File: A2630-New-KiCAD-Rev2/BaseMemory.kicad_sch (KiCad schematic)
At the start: 13 parts, among them U300 74HCT05, U400 SDRAM_32Mb(2Mx16), U401 SDRAM_32Mb(2Mx16), U606 74HCT244

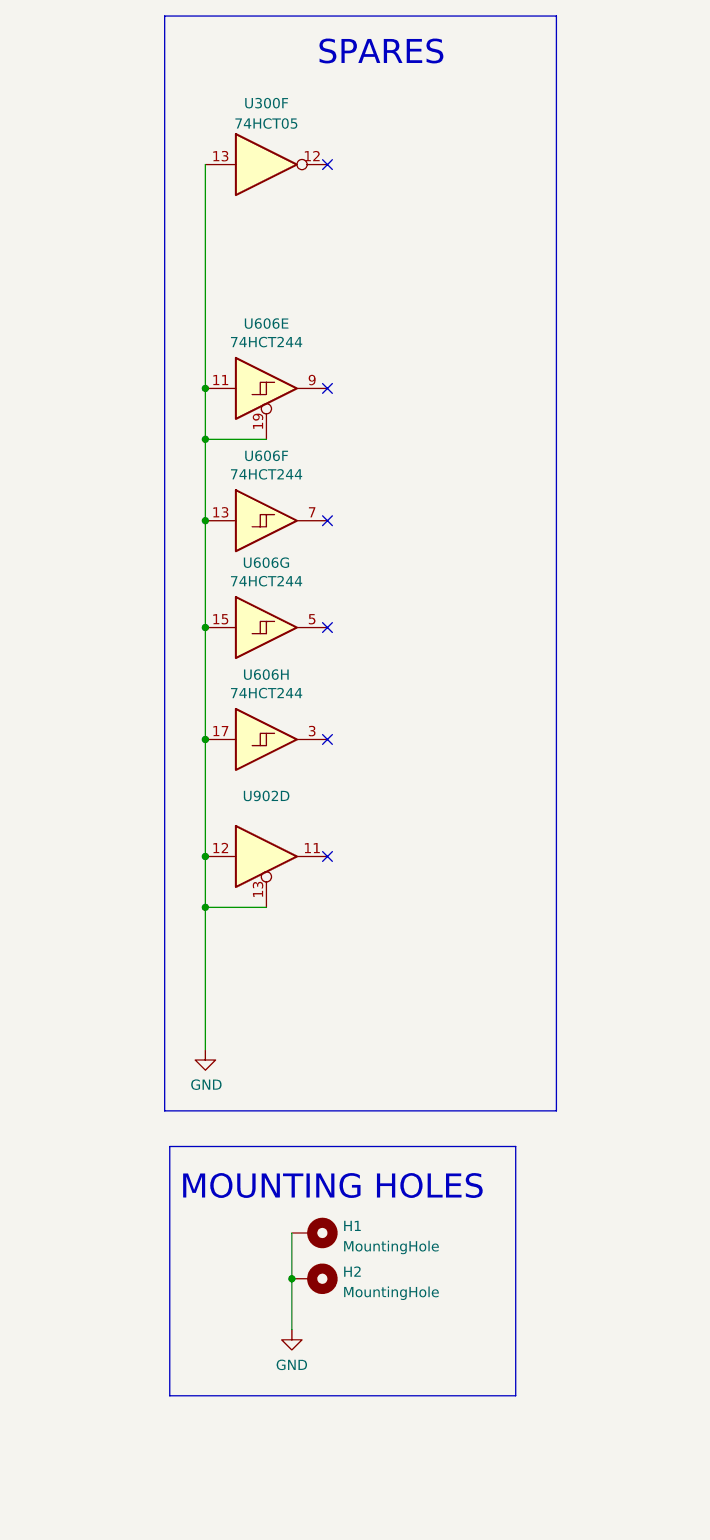
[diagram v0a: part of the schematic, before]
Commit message: Add files via upload
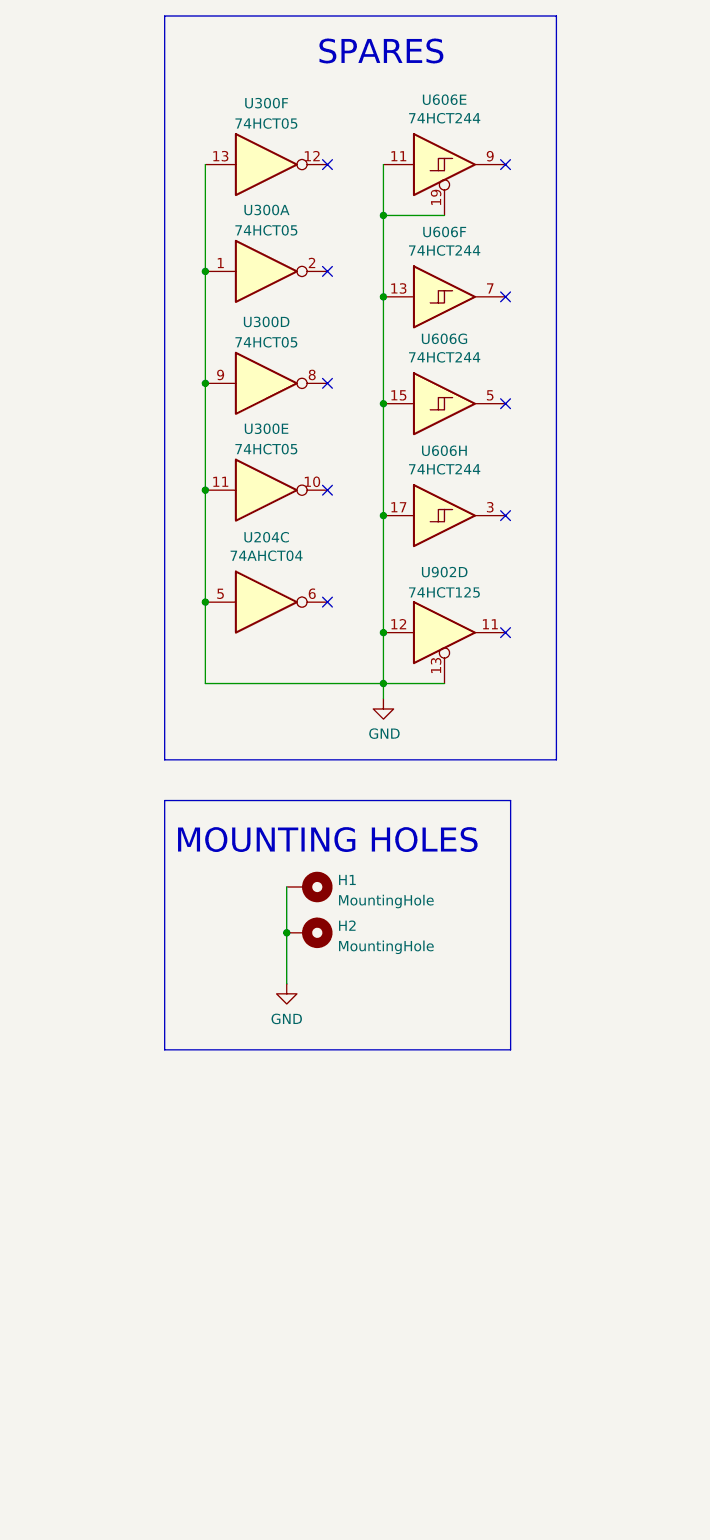
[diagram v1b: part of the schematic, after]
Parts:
- added U204: 74AHCT04, Package_SO:SOIC-14_3.9x8.7mm_P1.27mm, symbol 74xx:74HCT04
- added unit 1 of U300
- added unit 4 of U300
- added unit 5 of U300
- U902: value (none) -> 74HCT125; footprint (none) -> Package_SO:SOIC-14_3.9x8.7mm_P1.27mm
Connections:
- net GND: now also U204.5, U300.1, U300.11, U300.9
- no-connect marks 6 -> 10
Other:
- moved on the sheet: H1, H2, U606E, U606F, U606G, U606H, U902D
